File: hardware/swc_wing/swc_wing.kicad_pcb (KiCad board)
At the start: 2 copper layers, 62.8 x 58.7 mm, 53 parts, among them J1 Conn_01x06_Female, J2 Conn_01x05, J3 Conn_01x06_Female, J4 Conn_01x01_Female, Q1 2N7002, Q2 2N7002, Q3 2N7002, Q4 2N7002, Q5 2N7002, SW1 SW_Push_LED, SW2 SW_Push_LED, SW3 SW_Push_LED, SW4 SW_Push_LED, SW5 SW_Push_LED, U1 PCA9557PW, U2 PCA9557PW, U3 PCA9557PW

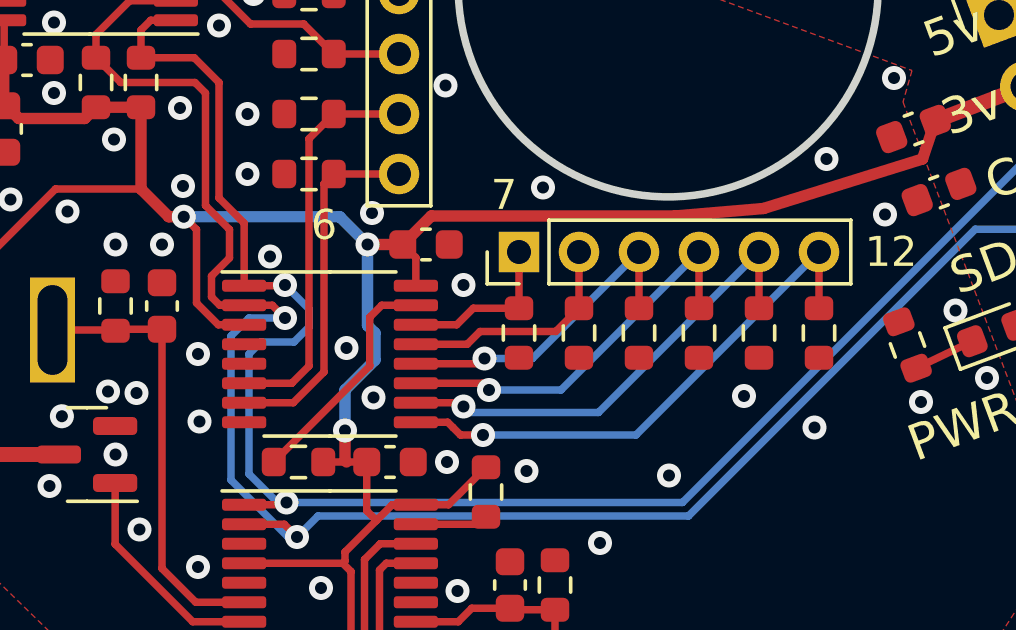
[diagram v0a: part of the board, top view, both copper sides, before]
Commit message: wing drc
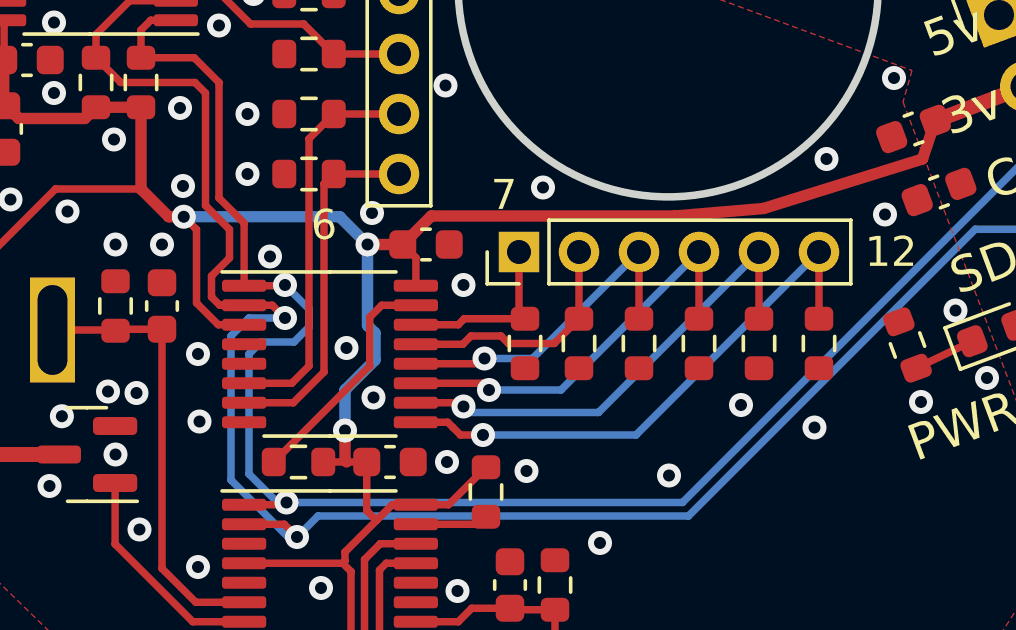
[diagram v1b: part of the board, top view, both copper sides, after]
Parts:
- moved R18 0.40 mm to (54.2, 91.0)
- moved R19 0.35 mm to (56.0, 91.0)
- moved R20 0.35 mm to (58.0, 91.0)
- moved R21 0.35 mm to (60.0, 91.0)
- moved R22 0.35 mm to (62.0, 91.0)
- moved R23 0.35 mm to (64.0, 91.0)
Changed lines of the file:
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@@
   (net 38 "Net-(Q1-Pad3)")
   (footprint "Resistor_SMD:R_0603_1608Metric" (layer "F.Cu")
-    (at 62 90.6 90)
+    (at 62 90.95 90)
     (descr "Resistor SMD 0603 (1608 Metric), square (rectangular) end terminal, IPC_7351 nominal, (Body size source: IPC-SM-782 page 72, https://www.pcb-3d.com/wordpress/wp-content/uploads/ipc-sm-782a_amendment_1_and_2.pdf), generated with kicad-footprint-generator")
     (tags "resistor")
@@
   )
   (footprint "Resistor_SMD:R_0603_1608Metric" (layer "F.Cu")
-    (at 58 90.6 90)
+    (at 58 90.95 90)
     (descr "Resistor SMD 0603 (1608 Metric), square (rectangular) end terminal, IPC_7351 nominal, (Body size source: IPC-SM-782 page 72, https://www.pcb-3d.com/wordpress/wp-content/uploads/ipc-sm-782a_amendment_1_and_2.pdf), generated with kicad-footprint-generator")
     (tags "resistor")
@@
   )
   (footprint "Resistor_SMD:R_0603_1608Metric" (layer "F.Cu")
-    (at 54 90.6 90)
+    (at 54.2 90.95 90)
     (descr "Resistor SMD 0603 (1608 Metric), square (rectangular) end terminal, IPC_7351 nominal, (Body size source: IPC-SM-782 page 72, https://www.pcb-3d.com/wordpress/wp-content/uploads/ipc-sm-782a_amendment_1_and_2.pdf), generated with kicad-footprint-generator")
     (tags "resistor")
@@
   )
   (footprint "Resistor_SMD:R_0603_1608Metric" (layer "F.Cu")
-    (at 60 90.6 90)
+    (at 60 90.95 90)
     (descr "Resistor SMD 0603 (1608 Metric), square (rectangular) end terminal, IPC_7351 nominal, (Body size source: IPC-SM-782 page 72, https://www.pcb-3d.com/wordpress/wp-content/uploads/ipc-sm-782a_amendment_1_and_2.pdf), generated with kicad-footprint-generator")
     (tags "resistor")
@@
   )
   (footprint "Resistor_SMD:R_0603_1608Metric" (layer "F.Cu")
-    (at 56 90.6 90)
+    (at 56 90.95 90)
     (descr "Resistor SMD 0603 (1608 Metric), square (rectangular) end terminal, IPC_7351 nominal, (Body size source: IPC-SM-782 page 72, https://www.pcb-3d.com/wordpress/wp-content/uploads/ipc-sm-782a_amendment_1_and_2.pdf), generated with kicad-footprint-generator")
     (tags "resistor")
@@
   )
   (footprint "Resistor_SMD:R_0603_1608Metric" (layer "F.Cu")
-    (at 64 90.6 90)
+    (at 64 90.95 90)
     (descr "Resistor SMD 0603 (1608 Metric), square (rectangular) end terminal, IPC_7351 nominal, (Body size source: IPC-SM-782 page 72, https://www.pcb-3d.com/wordpress/wp-content/uploads/ipc-sm-782a_amendment_1_and_2.pdf), generated with kicad-footprint-generator")
     (tags "resistor")
@@
   (via (at 42.7 83.1) (size 0.8) (drill 0.4) (layers "F.Cu" "B.Cu") (net 2))
   (via (at 51.6 94.9) (size 0.8) (drill 0.4) (layers "F.Cu" "B.Cu") (net 2))
-  (via (at 61.5 92.7) (size 0.8) (drill 0.4) (layers "F.Cu" "B.Cu") (net 2))
+  (via (at 61.4 93) (size 0.8) (drill 0.4) (layers "F.Cu" "B.Cu") (net 2))
   (via (at 41.140943 70.132385) (size 0.8) (drill 0.4) (layers "F.Cu" "B.Cu") (net 2))
   (via (at 45.25 77.3) (size 0.8) (drill 0.4) (layers "F.Cu" "B.Cu") (net 2))
@@
   (via (at 42.825 86.725) (size 0.8) (drill 0.4) (layers "F.Cu" "B.Cu") (net 12))
   (segment (start 65.8 103.25) (end 67.85 105.3) (width 0.25) (layer "B.Cu") (net 12))
-  (segment (start 43 86.9) (end 42.825 86.725) (width 0.25) (layer "B.Cu") (net 12))
   (segment (start 36.490075 64.290075) (end 36.490075 63.77753) (width 0.25) (layer "B.Cu") (net 12))
   (segment (start 48.95 90.35) (end 48.95 87.65) (width 0.38) (layer "B.Cu") (net 12))
@@
   (segment (start 51.625 93.575) (end 51.8 93.75) (width 0.25) (layer "F.Cu") (net 32))
   (segment (start 50.5625 93.575) (end 51.625 93.575) (width 0.25) (layer "F.Cu") (net 32))
-  (segment (start 64 89.775) (end 64 87.9) (width 0.25) (layer "F.Cu") (net 32))
   (segment (start 52.05 94) (end 52.8 94) (width 0.25) (layer "F.Cu") (net 32))
   (segment (start 51.8 93.75) (end 52.05 94) (width 0.25) (layer "F.Cu") (net 32))
+  (segment (start 64 87.9) (end 64 90.125) (width 0.25) (layer "F.Cu") (net 32))
   (via (at 52.8 94) (size 0.8) (drill 0.4) (layers "F.Cu" "B.Cu") (net 32))
   (segment (start 52.8 94) (end 57.9 94) (width 0.25) (layer "B.Cu") (net 32))
   (segment (start 57.9 94) (end 64 87.9) (width 0.25) (layer "B.Cu") (net 32))
-  (segment (start 62 87.9) (end 62 89.775) (width 0.25) (layer "F.Cu") (net 33))
   (segment (start 50.5625 92.925) (end 52.025 92.925) (width 0.25) (layer "F.Cu") (net 33))
   (segment (start 52.025 92.925) (end 52.15 93.05) (width 0.25) (layer "F.Cu") (net 33))
+  (segment (start 62 87.9) (end 62 90.125) (width 0.25) (layer "F.Cu") (net 33))
   (via (at 52.15 93.05) (size 0.8) (drill 0.4) (layers "F.Cu" "B.Cu") (net 33))
   (segment (start 56.65 93.25) (end 62 87.9) (width 0.25) (layer "B.Cu") (net 33))
@@
   (segment (start 50.5625 92.275) (end 52.775 92.275) (width 0.25) (layer "F.Cu") (net 34))
   (segment (start 52.775 92.275) (end 53 92.5) (width 0.25) (layer "F.Cu") (net 34))
-  (segment (start 60 87.9) (end 60 89.775) (width 0.25) (layer "F.Cu") (net 34))
+  (segment (start 60 87.9) (end 60 90.125) (width 0.25) (layer "F.Cu") (net 34))
   (via (at 53 92.5) (size 0.8) (drill 0.4) (layers "F.Cu" "B.Cu") (net 34))
   (segment (start 55.4 92.5) (end 60 87.9) (width 0.25) (layer "B.Cu") (net 34))
   (segment (start 53 92.5) (end 55.4 92.5) (width 0.25) (layer "B.Cu") (net 34))
-  (segment (start 58 87.9) (end 58 89.775) (width 0.25) (layer "F.Cu") (net 35))
+  (segment (start 58 87.9) (end 58 90.125) (width 0.25) (layer "F.Cu") (net 35))
   (segment (start 50.5625 91.625) (end 52.675 91.625) (width 0.25) (layer "F.Cu") (net 35))
   (segment (start 52.675 91.625) (end 52.85 91.45) (width 0.25) (layer "F.Cu") (net 35))
@@
   (segment (start 54.45 91.45) (end 58 87.9) (width 0.25) (layer "B.Cu") (net 35))
   (segment (start 52.85 91.45) (end 54.45 91.45) (width 0.25) (layer "B.Cu") (net 35))
-  (segment (start 52.7 90.55) (end 52.275 90.975) (width 0.25) (layer "F.Cu") (net 36))
-  (segment (start 56 89.775) (end 55.225 90.55) (width 0.25) (layer "F.Cu") (net 36))
-  (segment (start 55.225 90.55) (end 52.7 90.55) (width 0.25) (layer "F.Cu") (net 36))
-  (segment (start 56 89.775) (end 56 87.9) (width 0.25) (layer "F.Cu") (net 36))
-  (segment (start 52.275 90.975) (end 50.5625 90.975) (width 0.25) (layer "F.Cu") (net 36))
-  (segment (start 54 87.9) (end 54 89.775) (width 0.25) (layer "F.Cu") (net 37))
-  (segment (start 50.5625 90.325) (end 51.925 90.325) (width 0.25) (layer "F.Cu") (net 37))
-  (segment (start 52.475 89.775) (end 54 89.775) (width 0.25) (layer "F.Cu") (net 37))
-  (segment (start 51.925 90.325) (end 52.475 89.775) (width 0.25) (layer "F.Cu") (net 37))
+  (segment (start 52.4 90.7) (end 53.4 90.7) (width 0.25) (layer "F.Cu") (net 36))
+  (segment (start 53.65 90.95) (end 55.175 90.95) (width 0.25) (layer "F.Cu") (net 36))
+  (segment (start 55.175 90.95) (end 56 90.125) (width 0.25) (layer "F.Cu") (net 36))
+  (segment (start 50.5625 90.975) (end 52.125 90.975) (width 0.25) (layer "F.Cu") (net 36))
+  (segment (start 53.4 90.7) (end 53.65 90.95) (width 0.25) (layer "F.Cu") (net 36))
+  (segment (start 56 90.125) (end 56 87.9) (width 0.25) (layer "F.Cu") (net 36))
+  (segment (start 52.125 90.975) (end 52.4 90.7) (width 0.25) (layer "F.Cu") (net 36))
+  (segment (start 54 87.9) (end 54 89.925) (width 0.25) (layer "F.Cu") (net 37))
+  (segment (start 52.175 90.125) (end 51.975 90.325) (width 0.25) (layer "F.Cu") (net 37))
+  (segment (start 54 89.925) (end 54.2 90.125) (width 0.25) (layer "F.Cu") (net 37))
+  (segment (start 51.975 90.325) (end 50.5625 90.325) (width 0.25) (layer "F.Cu") (net 37))
+  (segment (start 54.2 90.125) (end 52.175 90.125) (width 0.25) (layer "F.Cu") (net 37))
   (segment (start 38.9 67.5625) (end 38.9 66.6) (width 0.25) (layer "F.Cu") (net 38))
   (segment (start 40.622957 64.877043) (end 41.449659 64.877043) (width 0.25) (layer "F.Cu") (net 38))
